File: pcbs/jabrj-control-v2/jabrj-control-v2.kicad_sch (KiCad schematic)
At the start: 11 parts

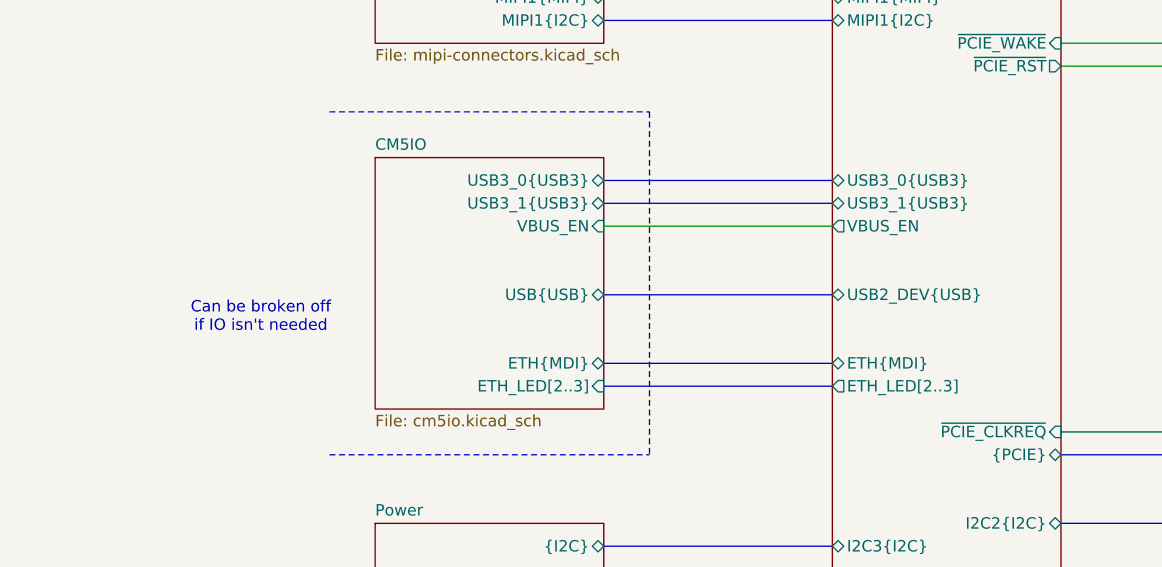
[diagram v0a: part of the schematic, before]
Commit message: 400 Unrouted
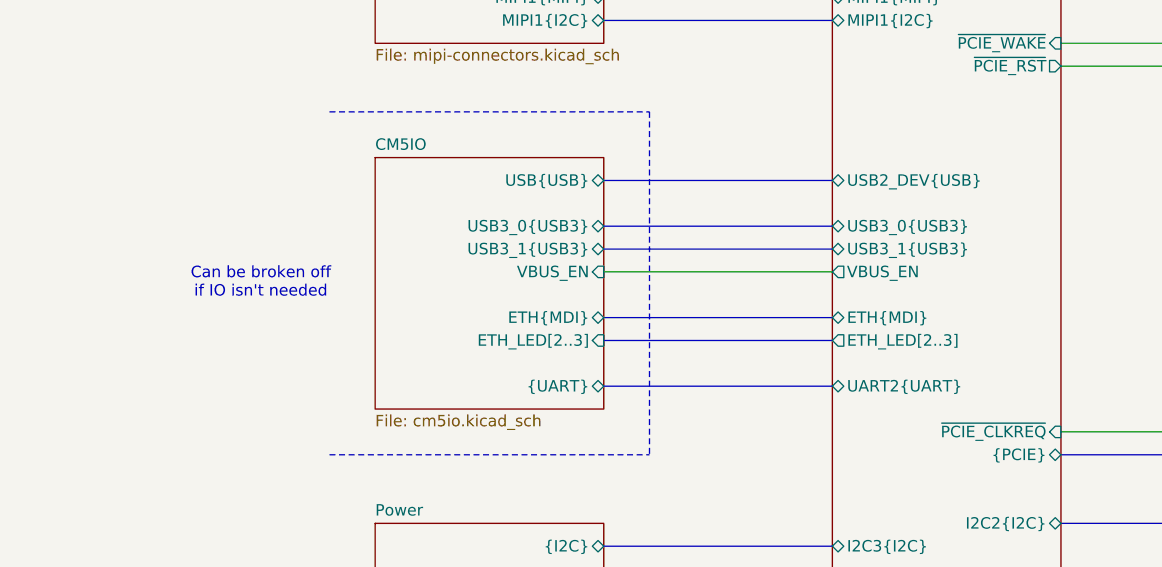
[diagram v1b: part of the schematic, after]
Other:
- sheet CM5 ports: added UART2{UART}; removed none
- sheet CM5IO ports: added {UART}; removed none
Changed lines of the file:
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@@
 	(text "Can be broken off\nif IO isn't needed"
 		(exclude_from_sim no)
-		(at 58.42 81.28 0)
+		(at 58.42 77.47 0)
 		(effects
 			(font
@@
 	(bus
 		(pts
-			(xy 96.52 66.04) (xy 121.92 66.04)
+			(xy 96.52 71.12) (xy 121.92 71.12)
 		)
 		(stroke
@@
 	(bus
 		(pts
-			(xy 96.52 86.36) (xy 121.92 86.36)
+			(xy 96.52 81.28) (xy 121.92 81.28)
 		)
 		(stroke
@@
 	(bus
 		(pts
-			(xy 96.52 78.74) (xy 121.92 78.74)
+			(xy 96.52 66.04) (xy 121.92 66.04)
 		)
 		(stroke
@@
 	(bus
 		(pts
-			(xy 96.52 88.9) (xy 121.92 88.9)
+			(xy 96.52 83.82) (xy 121.92 83.82)
 		)
 		(stroke
@@
 	(bus
 		(pts
-			(xy 96.52 68.58) (xy 121.92 68.58)
+			(xy 96.52 73.66) (xy 121.92 73.66)
 		)
 		(stroke
@@
 	(wire
 		(pts
-			(xy 96.52 71.12) (xy 121.92 71.12)
+			(xy 96.52 76.2) (xy 121.92 76.2)
 		)
 		(stroke
@@
 		)
 	)
+	(bus
+		(pts
+			(xy 96.52 88.9) (xy 121.92 88.9)
+		)
+		(stroke
+			(width 0)
+			(type default)
+		)
+	)
 	(polyline
 		(pts
@@
 		)
 		(pin "ETH_LED[2..3]" output
-			(at 121.92 88.9 180)
+			(at 121.92 83.82 180)
 			(effects
 				(font
@@
 		)
 		(pin "ETH{MDI}" bidirectional
-			(at 121.92 86.36 180)
+			(at 121.92 81.28 180)
 			(effects
 				(font
@@
 		)
 		(pin "VBUS_EN" output
-			(at 121.92 71.12 180)
+			(at 121.92 76.2 180)
 			(effects
 				(font
@@
 		)
 		(pin "USB2_DEV{USB}" bidirectional
-			(at 121.92 78.74 180)
+			(at 121.92 66.04 180)
 			(effects
 				(font
@@
 		)
 		(pin "USB3_0{USB3}" bidirectional
-			(at 121.92 66.04 180)
+			(at 121.92 71.12 180)
 			(effects
 				(font
@@
 		)
 		(pin "USB3_1{USB3}" bidirectional
-			(at 121.92 68.58 180)
+			(at 121.92 73.66 180)
 			(effects
 				(font
@@
 			)
 		)
+		(pin "UART2{UART}" bidirectional
+			(at 121.92 88.9 180)
+			(effects
+				(font
+					(size 1.27 1.27)
+				)
+				(justify left)
+			)
+		)
 		(instances
 			(project "jabrj-control-v2"
@@
 		)
 		(pin "ETH_LED[2..3]" input
-			(at 96.52 88.9 0)
+			(at 96.52 83.82 0)
 			(effects
 				(font
@@
 		)
 		(pin "ETH{MDI}" bidirectional
-			(at 96.52 86.36 0)
+			(at 96.52 81.28 0)
 			(effects
 				(font
@@
 		)
 		(pin "USB{USB}" bidirectional
-			(at 96.52 78.74 0)
+			(at 96.52 66.04 0)
 			(effects
 				(font
@@
 		)
 		(pin "USB3_0{USB3}" bidirectional
-			(at 96.52 66.04 0)
+			(at 96.52 71.12 0)
 			(effects
 				(font
@@
 		)
 		(pin "USB3_1{USB3}" bidirectional
-			(at 96.52 68.58 0)
+			(at 96.52 73.66 0)
 			(effects
 				(font
@@
 		)
 		(pin "VBUS_EN" input
-			(at 96.52 71.12 0)
+			(at 96.52 76.2 0)
+			(effects
+				(font
+					(size 1.27 1.27)
+				)
+				(justify right)
+			)
+		)
+		(pin "{UART}" bidirectional
+			(at 96.52 88.9 0)
 			(effects
 				(font
